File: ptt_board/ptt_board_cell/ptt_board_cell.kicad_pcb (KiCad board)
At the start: 2 copper layers, 62.4 x 27.8 mm, 7 parts, among them P019 Conn_01x01_Pin, P19 Conn_01x01_Pin

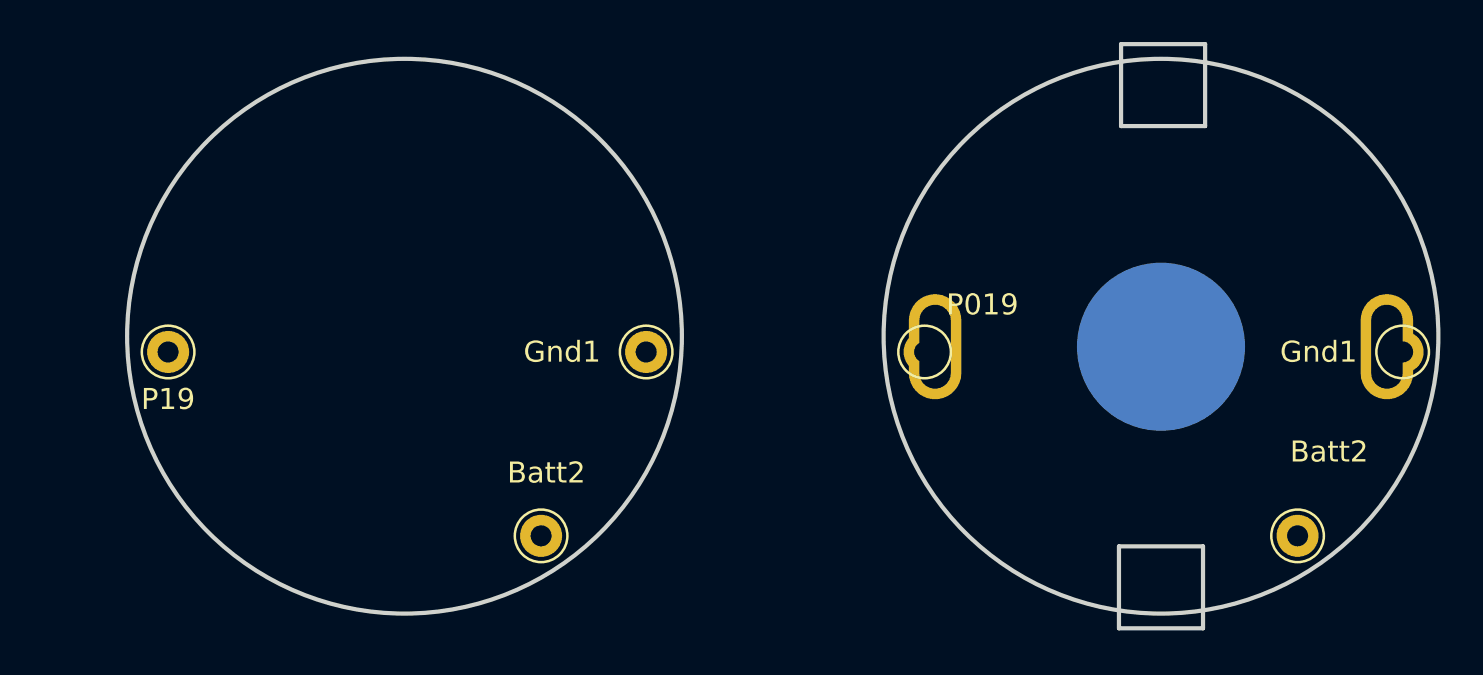
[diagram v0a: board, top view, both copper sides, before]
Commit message: [WIP]
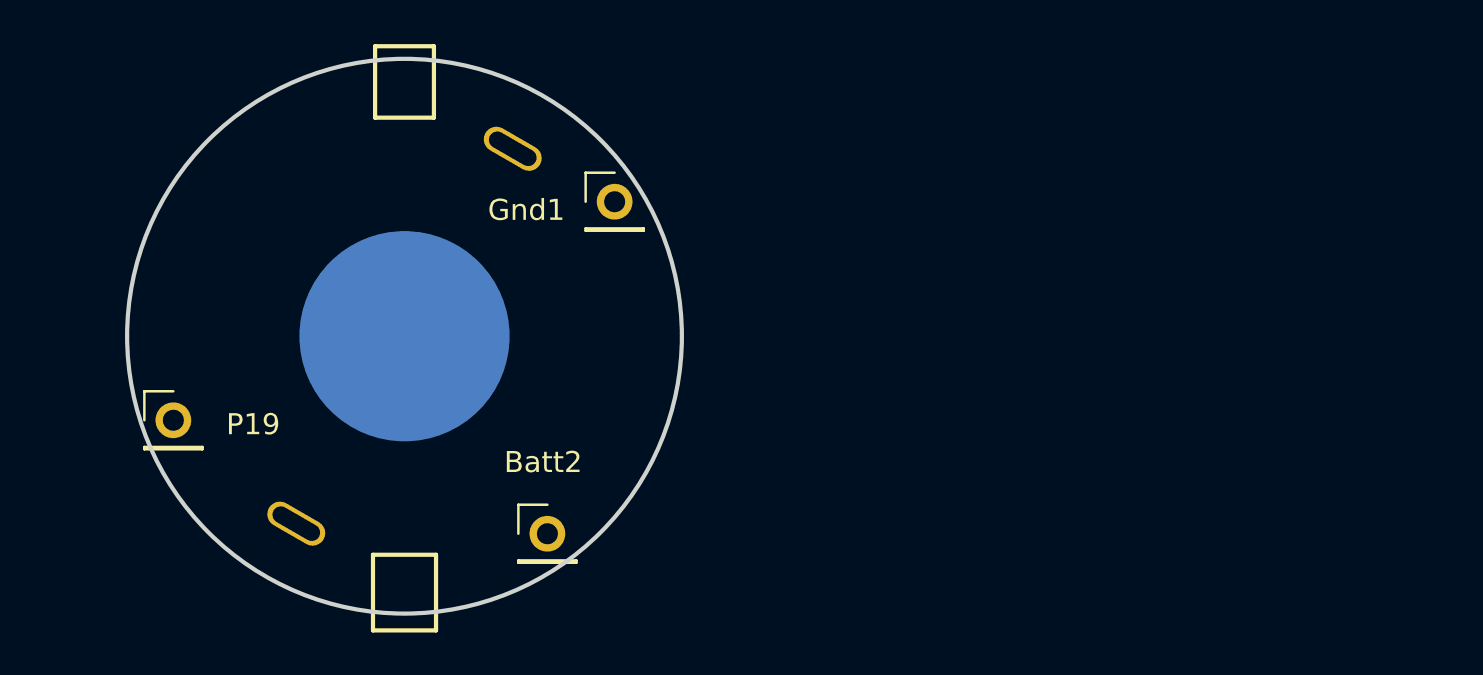
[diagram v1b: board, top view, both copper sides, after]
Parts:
- removed BAT1: MY-2032-22, Project_components:BAT-TH_MY-2032-22
- removed the Batt2 at (142.5, 109.5)
- removed the Batt2 at (106.5, 109.5)
- removed the Gnd1 at (111.5, 100.8)
- removed the Gnd1 at (147.5, 100.8)
- removed P019: Conn_01x01_Pin, Connector_Pin:Pin_D1.0mm_L10.0mm
- added Batt2: Conn_01x01_Pin, Connector_PinHeader_2.54mm:PinHeader_1x01_P2.54mm_Vertical, F.Cu at (106.8, 109.4)
- added Gnd1: Conn_01x01_Pin, Connector_PinHeader_2.54mm:PinHeader_1x01_P2.54mm_Vertical, F.Cu at (110.0, 93.6)
- added U1: MY-2032-02, Project_components:BATT-TH_MY-2032-02, B.Cu at (100.0, 100.0)
- P19: footprint Connector_Pin:Pin_D1.0mm_L10.0mm -> Connector_PinHeader_2.54mm:PinHeader_1x01_P2.54mm_Vertical
- moved P19 3.26 mm to (89.0, 104.0)
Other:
- board size 62.4 x 27.8 mm -> 26.4 x 26.4 mm

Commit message: [WIP]
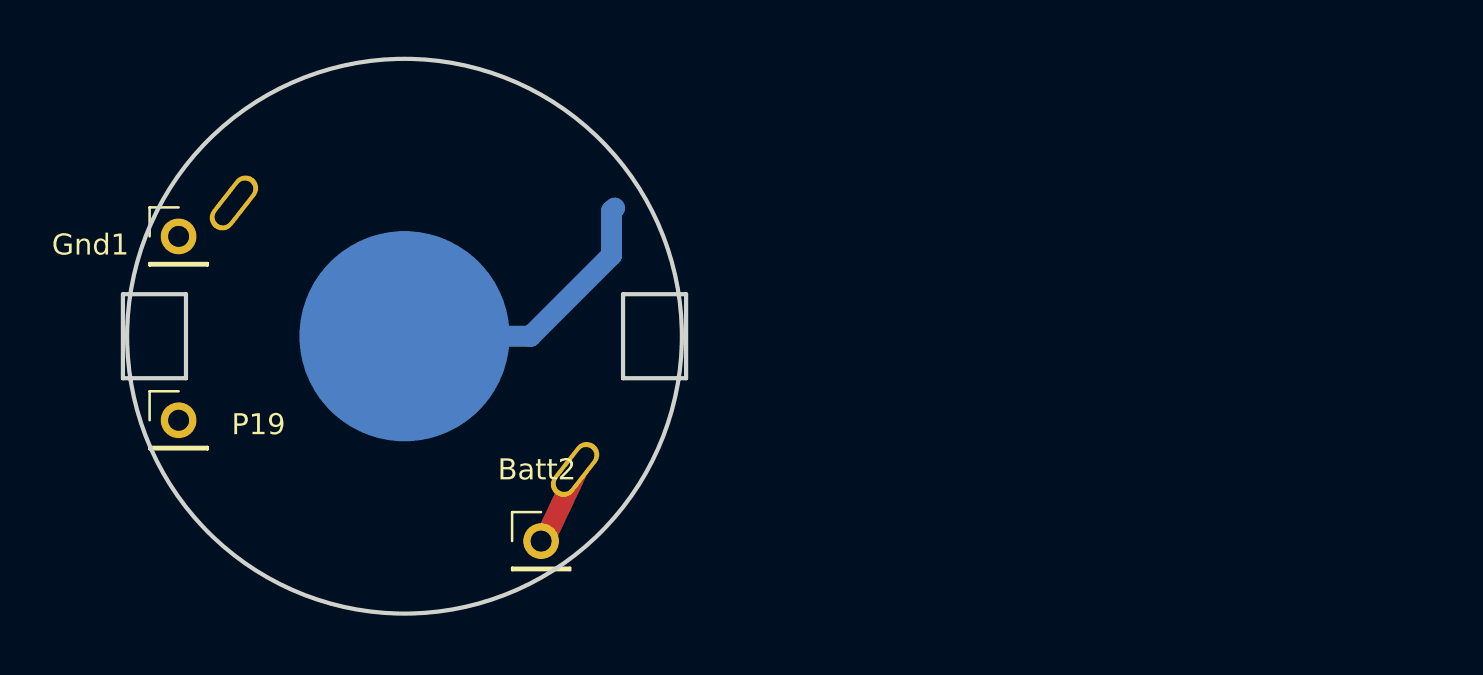
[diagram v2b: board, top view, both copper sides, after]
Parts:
- moved Gnd1 20.8 mm to (89.2, 95.2)
- moved Batt2 0.46 mm to (106.5, 109.8)
- moved P19 0.25 mm to (89.2, 104.0)
- turned U1 to -38 degrees
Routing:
- net GND: track 0.00 -> 14.0 mm
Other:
- board size 26.4 x 26.4 mm -> 26.8 x 26.4 mm
- board text added: "Gnd1"

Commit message: [Housekeeping] Renamed project library
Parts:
- U1: footprint Project_components:BATT-TH_MY-2032-02 -> PTT_Project_library:BATT-TH_MY-2032-02
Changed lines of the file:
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@@
 		)
 	)
-	(footprint "Project_components:BATT-TH_MY-2032-02"
+	(footprint "PTT_Project_library:BATT-TH_MY-2032-02"
 		(layer "B.Cu")
 		(at 100 100 -38)
@@
 		)
 		(embedded_fonts no)
-		(model "/home/rbaruffa/Perso/OmniPTT/hardware/libraries/Project_components.3dshapes/BATT-TH_MY-2032-02.wrl"
+		(model "/home/rbaruffa/Perso/OmniPTT/hardware/libraries/PTT_Project_library.3dshapes/BATT-TH_MY-2032-02.wrl"
 			(offset
 				(xyz 0 0 0)
